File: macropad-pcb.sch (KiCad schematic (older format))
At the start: 24 parts, among them SW1 SW_Push, U1 ATmega32U4-AU, Y1 16MHz

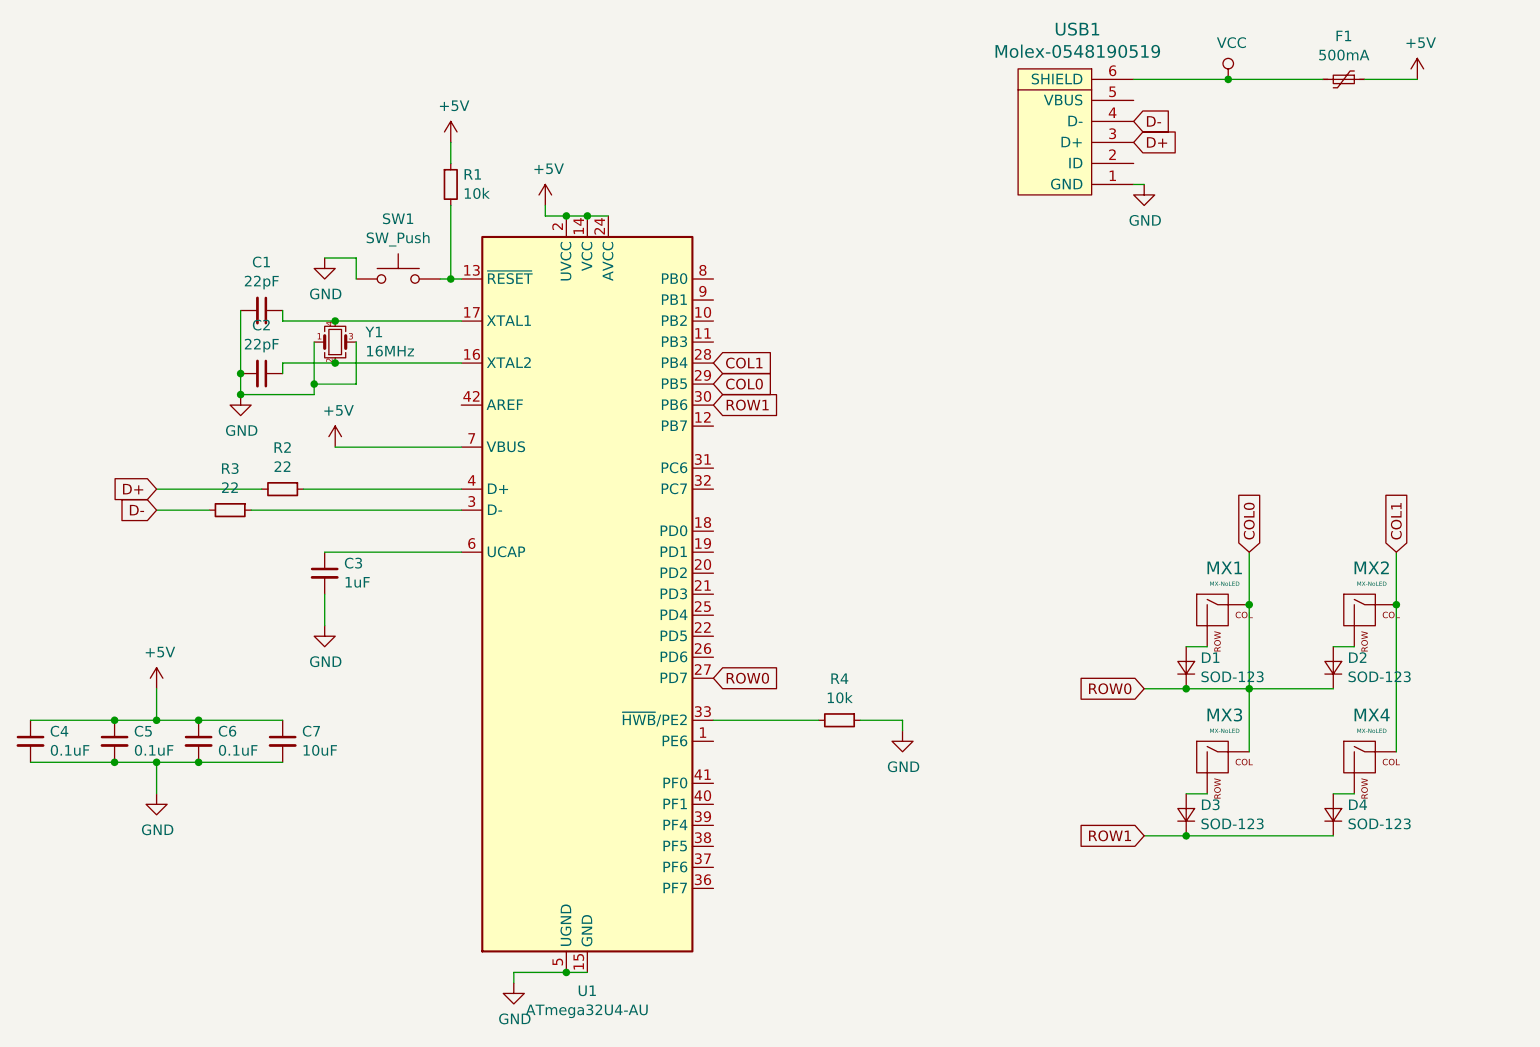
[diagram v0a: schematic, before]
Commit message: finalise schematic
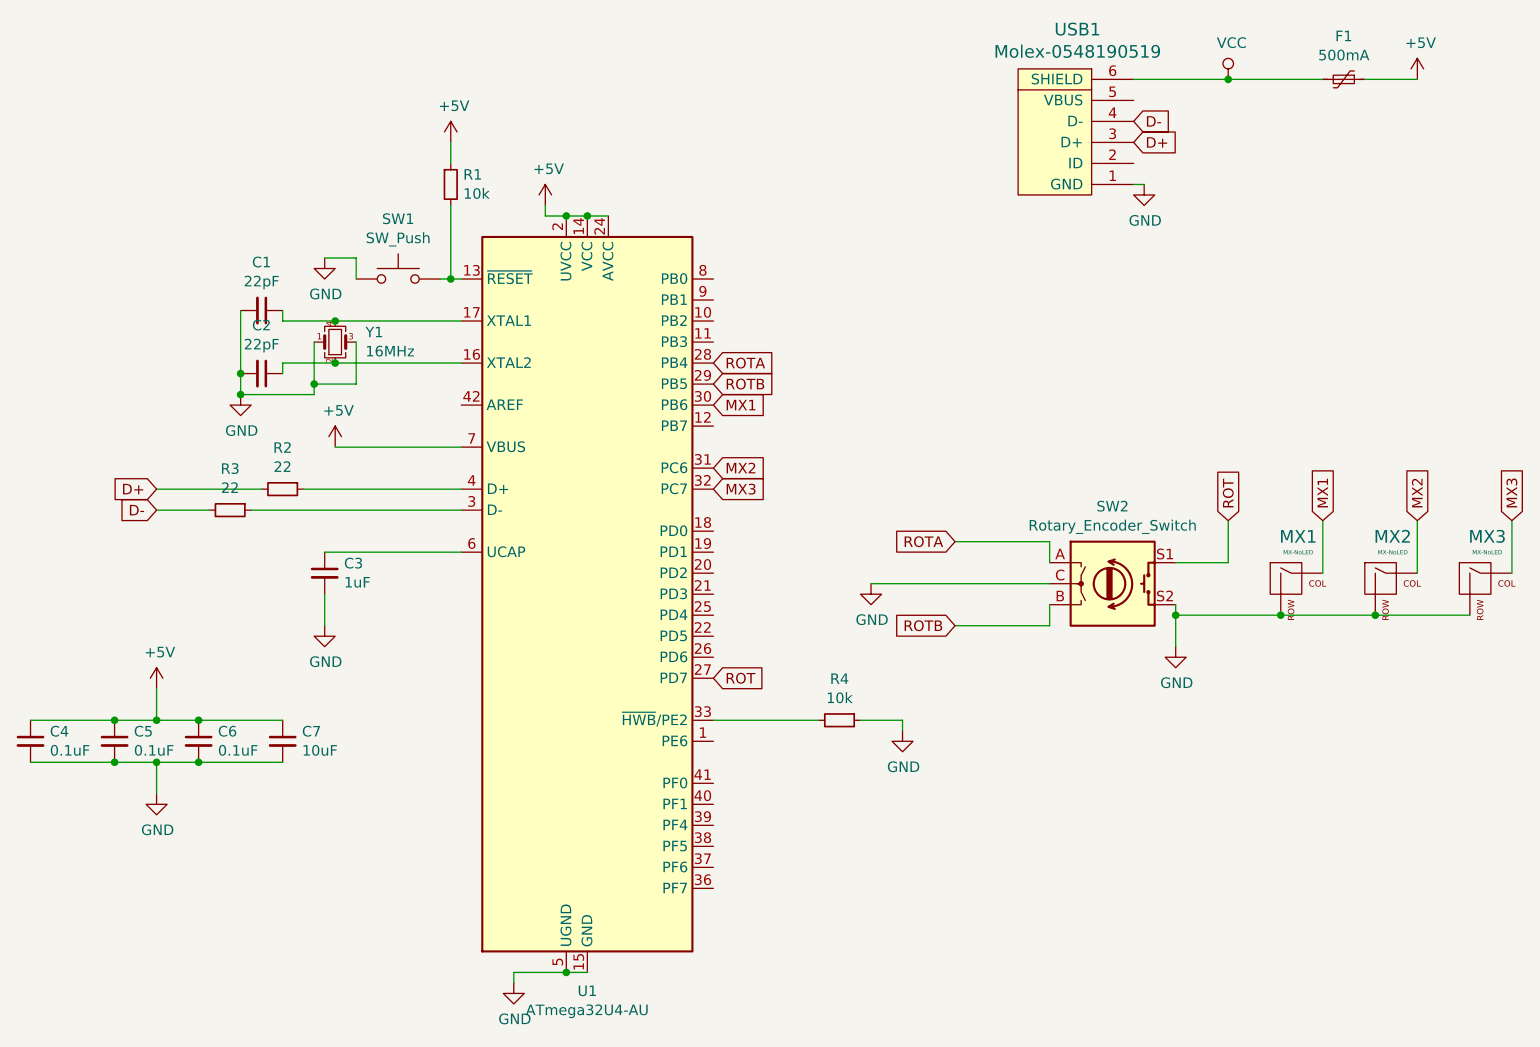
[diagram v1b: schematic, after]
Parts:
- removed D1, D2, D3, D4: SOD-123, Diode_SMD:D_SOD-123, symbol Device:D_Small
- removed MX4: MX-NoLED, symbol MX_Alps_Hybrid:MX-NoLED
- added SW2: Rotary_Encoder_Switch, Rotary_Encoder:RotaryEncoder_Alps_EC11E-Switch_Vertical_H20mm, symbol Device:Rotary_Encoder_Switch
- MX1, MX2, MX3: footprint (none) -> MX_Alps_Hybrid:MX-1U-NoLED
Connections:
- net GND: now also MX1.2 (ROW), MX2.2 (ROW), MX3.2 (ROW), SW2.C, SW2.S2
- net MX2: now reaches U1.31 (PC6)
- net MX2: now also MX2.1 (COL)
- net MX3: now reaches U1.32 (PC7)
- net MX3: now also MX3.1 (COL)
- removed net COL0: MX1.1 (COL), MX3.1 (COL), U1.27 (PD7), U1.29 (PB5)
- net COL1 renamed ROTA
- net ROTA: now also SW2.A; no longer MX2.1 (COL)
- net ROW1 renamed MX1
- net MX1: now also MX1.1 (COL)
- new net ROT: SW2.S1, U1.27 (PD7)
- new net ROTB: SW2.B, U1.29 (PB5)
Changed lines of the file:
@@
 EESchema Schematic File Version 4
+LIBS:macropad-pcb-cache
 EELAYER 30 0
 EELAYER END
@@
 	8400 2000 8350 2000
 $Comp
+L Device:Rotary_Encoder_Switch SW2
+U 1 1 5F25C130
+P 8250 3900
+F 0 "SW2" H 8250 4267 50  0000 C CNN
+F 1 "Rotary_Encoder_Switch" H 8250 4176 50  0000 C CNN
+F 2 "Rotary_Encoder:RotaryEncoder_Alps_EC11E-Switch_Vertical_H20mm" H 8100 4060 50  0001 C CNN
+F 3 "~" H 8250 4160 50  0001 C CNN
+	1    8250 3900
+	1    0    0    -1
+$EndComp
+$Comp
 L MX_Alps_Hybrid:MX-NoLED MX1
-U 1 1 5F291437
-P 8750 4050
-F 0 "MX1" H 8783 4273 60  0000 C CNN
-F 1 "MX-NoLED" H 8783 4199 20  0000 C CNN
-F 2 "" H 8125 4025 60  0001 C CNN
-F 3 "" H 8125 4025 60  0001 C CNN
-	1    8750 4050
-	1    0    0    -1
-$EndComp
-$Comp
-L Device:D_Small D1
-U 1 1 5F2925B5
-P 8600 4300
-F 0 "D1" V 8646 4232 50  0000 R CNN
-F 1 "SOD-123" V 8555 4232 50  0000 R CNN
-F 2 "Diode_SMD:D_SOD-123" V 8600 4300 50  0001 C CNN
-F 3 "~" V 8600 4300 50  0001 C CNN
-	1    8600 4300
-	0    -1   -1   0
-$EndComp
-Wire Wire Line
-	8600 4200 8700 4200
+U 1 1 5F26C0EC
+P 9100 3900
+F 0 "MX1" H 9133 4123 60  0000 C CNN
+F 1 "MX-NoLED" H 9133 4049 20  0000 C CNN
+F 2 "MX_Alps_Hybrid:MX-1U-NoLED" H 8475 3875 60  0001 C CNN
+F 3 "" H 8475 3875 60  0001 C CNN
+	1    9100 3900
+	1    0    0    -1
+$EndComp
 $Comp
 L MX_Alps_Hybrid:MX-NoLED MX2
-U 1 1 5F29D570
-P 9450 4050
-F 0 "MX2" H 9483 4273 60  0000 C CNN
-F 1 "MX-NoLED" H 9483 4199 20  0000 C CNN
-F 2 "" H 8825 4025 60  0001 C CNN
-F 3 "" H 8825 4025 60  0001 C CNN
-	1    9450 4050
-	1    0    0    -1
-$EndComp
-$Comp
-L Device:D_Small D2
-U 1 1 5F29D576
-P 9300 4300
-F 0 "D2" V 9346 4232 50  0000 R CNN
-F 1 "SOD-123" V 9255 4232 50  0000 R CNN
-F 2 "Diode_SMD:D_SOD-123" V 9300 4300 50  0001 C CNN
-F 3 "~" V 9300 4300 50  0001 C CNN
-	1    9300 4300
-	0    -1   -1   0
-$EndComp
-Wire Wire Line
-	9300 4200 9400 4200
+U 1 1 5F26CAFC
+P 9550 3900
+F 0 "MX2" H 9583 4123 60  0000 C CNN
+F 1 "MX-NoLED" H 9583 4049 20  0000 C CNN
+F 2 "MX_Alps_Hybrid:MX-1U-NoLED" H 8925 3875 60  0001 C CNN
+F 3 "" H 8925 3875 60  0001 C CNN
+	1    9550 3900
+	1    0    0    -1
+$EndComp
 $Comp
 L MX_Alps_Hybrid:MX-NoLED MX3
-U 1 1 5F29F40F
-P 8750 4750
-F 0 "MX3" H 8783 4973 60  0000 C CNN
-F 1 "MX-NoLED" H 8783 4899 20  0000 C CNN
-F 2 "" H 8125 4725 60  0001 C CNN
-F 3 "" H 8125 4725 60  0001 C CNN
-	1    8750 4750
-	1    0    0    -1
-$EndComp
-$Comp
-L Device:D_Small D3
-U 1 1 5F29F415
-P 8600 5000
-F 0 "D3" V 8646 4932 50  0000 R CNN
-F 1 "SOD-123" V 8555 4932 50  0000 R CNN
-F 2 "Diode_SMD:D_SOD-123" V 8600 5000 50  0001 C CNN
-F 3 "~" V 8600 5000 50  0001 C CNN
-	1    8600 5000
-	0    -1   -1   0
-$EndComp
-Wire Wire Line
-	8600 4900 8700 4900
-$Comp
-L MX_Alps_Hybrid:MX-NoLED MX4
-U 1 1 5F2A1394
-P 9450 4750
-F 0 "MX4" H 9483 4973 60  0000 C CNN
-F 1 "MX-NoLED" H 9483 4899 20  0000 C CNN
-F 2 "" H 8825 4725 60  0001 C CNN
-F 3 "" H 8825 4725 60  0001 C CNN
-	1    9450 4750
-	1    0    0    -1
-$EndComp
-$Comp
-L Device:D_Small D4
-U 1 1 5F2A139A
-P 9300 5000
-F 0 "D4" V 9346 4932 50  0000 R CNN
-F 1 "SOD-123" V 9255 4932 50  0000 R CNN
-F 2 "Diode_SMD:D_SOD-123" V 9300 5000 50  0001 C CNN
-F 3 "~" V 9300 5000 50  0001 C CNN
-	1    9300 5000
-	0    -1   -1   0
-$EndComp
-Wire Wire Line
-	9300 4900 9400 4900
-Wire Wire Line
-	9300 4400 8900 4400
-Connection ~ 8600 4400
-Wire Wire Line
-	8600 4400 8400 4400
-Wire Wire Line
-	9300 5100 8600 5100
-Connection ~ 8600 5100
-Wire Wire Line
-	8600 5100 8400 5100
-Wire Wire Line
-	8900 3750 8900 4000
-Wire Wire Line
-	8900 4000 8900 4400
-Connection ~ 8900 4000
-Connection ~ 8900 4400
-Wire Wire Line
-	8900 4400 8600 4400
-Wire Wire Line
-	9600 4700 9600 4000
-Connection ~ 9600 4000
-Wire Wire Line
-	9600 4000 9600 3750
-Text GLabel 8900 3750 1    50   Input ~ 0
-COL0
-Text GLabel 9600 3750 1    50   Input ~ 0
-COL1
-Text GLabel 8400 4400 0    50   Input ~ 0
-ROW0
-Text GLabel 8400 5100 0    50   Input ~ 0
-ROW1
+U 1 1 5F26D0BB
+P 10000 3900
+F 0 "MX3" H 10033 4123 60  0000 C CNN
+F 1 "MX-NoLED" H 10033 4049 20  0000 C CNN
+F 2 "MX_Alps_Hybrid:MX-1U-NoLED" H 9375 3875 60  0001 C CNN
+F 3 "" H 9375 3875 60  0001 C CNN
+	1    10000 3900
+	1    0    0    -1
+$EndComp
+Wire Wire Line
+	7950 3700 7950 3800
+Wire Wire Line
+	7950 4000 7950 4100
+$Comp
+L power:GND #PWR0114
+U 1 1 5F28B8F7
+P 7100 3900
+F 0 "#PWR0114" H 7100 3650 50  0001 C CNN
+F 1 "GND" H 7105 3727 50  0000 C CNN
+F 2 "" H 7100 3900 50  0001 C CNN
+F 3 "" H 7100 3900 50  0001 C CNN
+	1    7100 3900
+	1    0    0    -1
+$EndComp
+Wire Wire Line
+	8550 4000 8550 4050
+Wire Wire Line
+	9250 3850 9250 3600
+Wire Wire Line
+	9700 3850 9700 3600
+Wire Wire Line
+	10150 3850 10150 3600
+Wire Wire Line
+	8550 3800 8800 3800
+Wire Wire Line
+	8800 3800 8800 3600
+Wire Wire Line
+	8550 4050 9050 4050
+Connection ~ 9050 4050
+Wire Wire Line
+	9050 4050 9500 4050
+Connection ~ 9500 4050
+Wire Wire Line
+	9500 4050 9950 4050
+Wire Wire Line
+	8550 4050 8550 4200
+Connection ~ 8550 4050
+$Comp
+L power:GND #PWR0115
+U 1 1 5F277CD8
+P 8550 4200
+F 0 "#PWR0115" H 8550 3950 50  0001 C CNN
+F 1 "GND" H 8555 4027 50  0000 C CNN
+F 2 "" H 8550 4200 50  0001 C CNN
+F 3 "" H 8550 4200 50  0001 C CNN
+	1    8550 4200
+	1    0    0    -1
+$EndComp
+Text GLabel 8800 3600 1    50   Input ~ 0
+ROT
+Text GLabel 9250 3600 1    50   Input ~ 0
+MX1
+Text GLabel 9700 3600 1    50   Input ~ 0
+MX2
+Text GLabel 10150 3600 1    50   Input ~ 0
+MX3
+Text GLabel 6350 4350 2    50   Input ~ 0
+ROT
+Text GLabel 6350 3050 2    50   Input ~ 0
+MX1
+Text GLabel 6350 3350 2    50   Input ~ 0
+MX2
+Text GLabel 6350 3450 2    50   Input ~ 0
+MX3
+Text GLabel 7500 3700 0    50   Input ~ 0
+ROTA
+Text GLabel 7500 4100 0    50   Input ~ 0
+ROTB
+Text GLabel 6350 2850 2    50   Input ~ 0
+ROTA
 Text GLabel 6350 2950 2    50   Input ~ 0
-COL0
-Text GLabel 6350 2850 2    50   Input ~ 0
-COL1
-Text GLabel 6350 4350 2    50   Input ~ 0
-ROW0
-Text GLabel 6350 3050 2    50   Input ~ 0
-ROW1
-Wire Wire Line
-	8900 4400 8900 4700
+ROTB
+Wire Wire Line
+	7500 3700 7950 3700
+Wire Wire Line
+	7100 3900 7950 3900
+Wire Wire Line
+	7500 4100 7950 4100
 $EndSCHEMATC
